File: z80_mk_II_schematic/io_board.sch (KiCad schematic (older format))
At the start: 3 parts

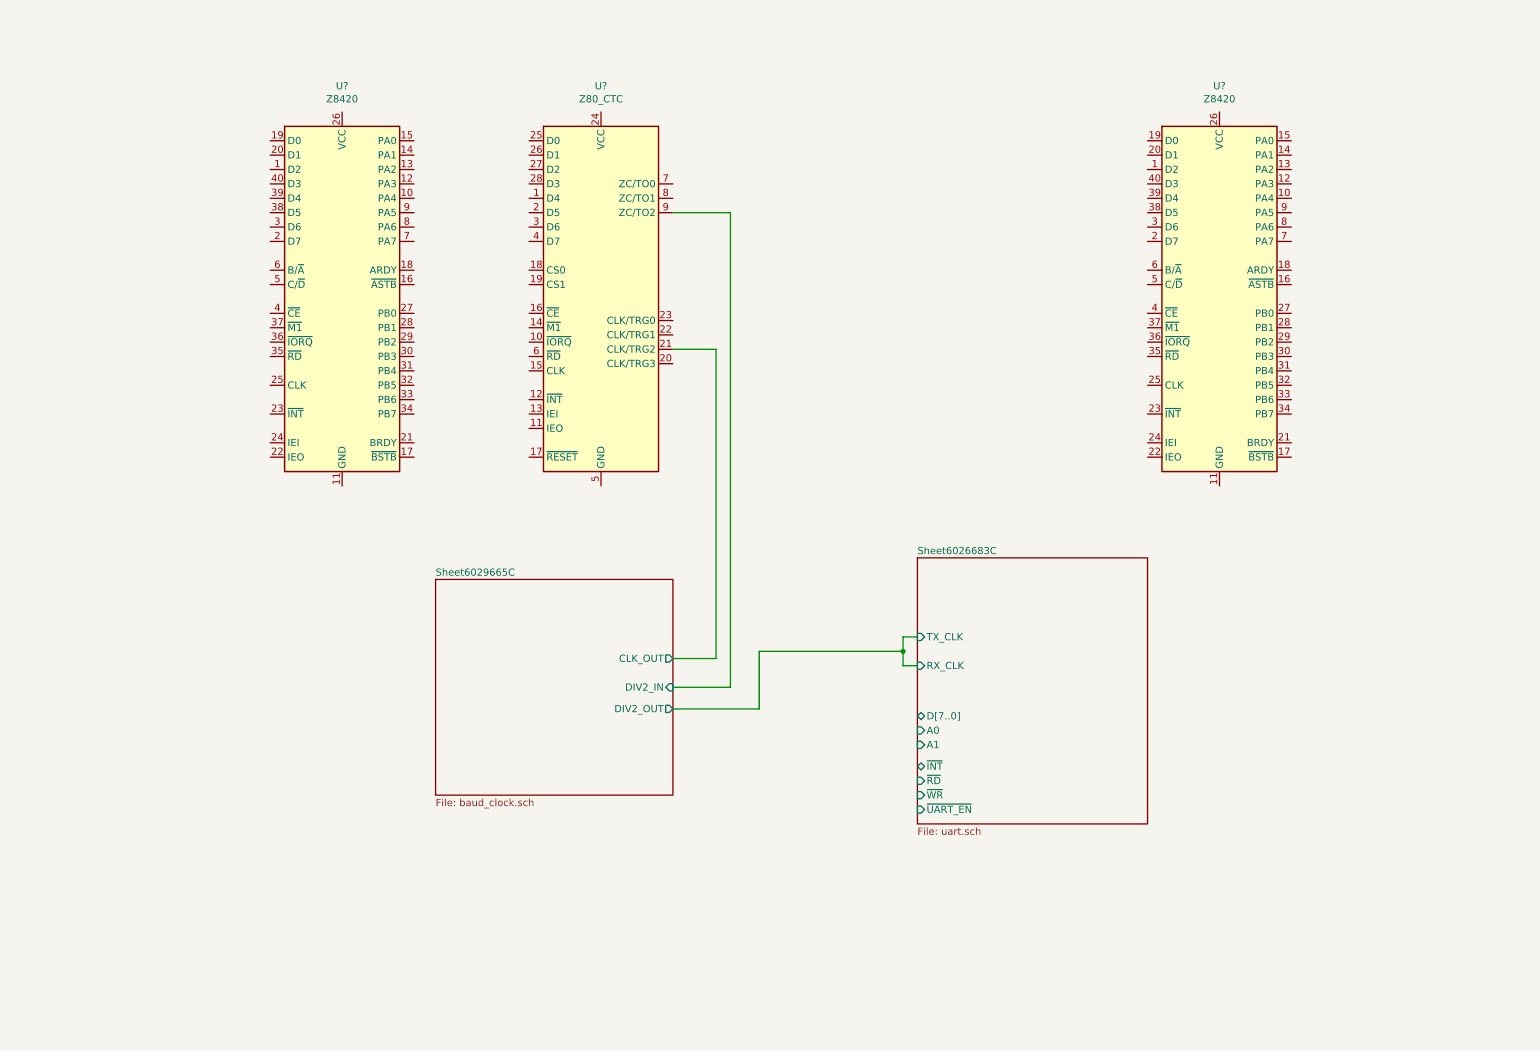
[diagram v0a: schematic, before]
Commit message: Lots more work on schematic
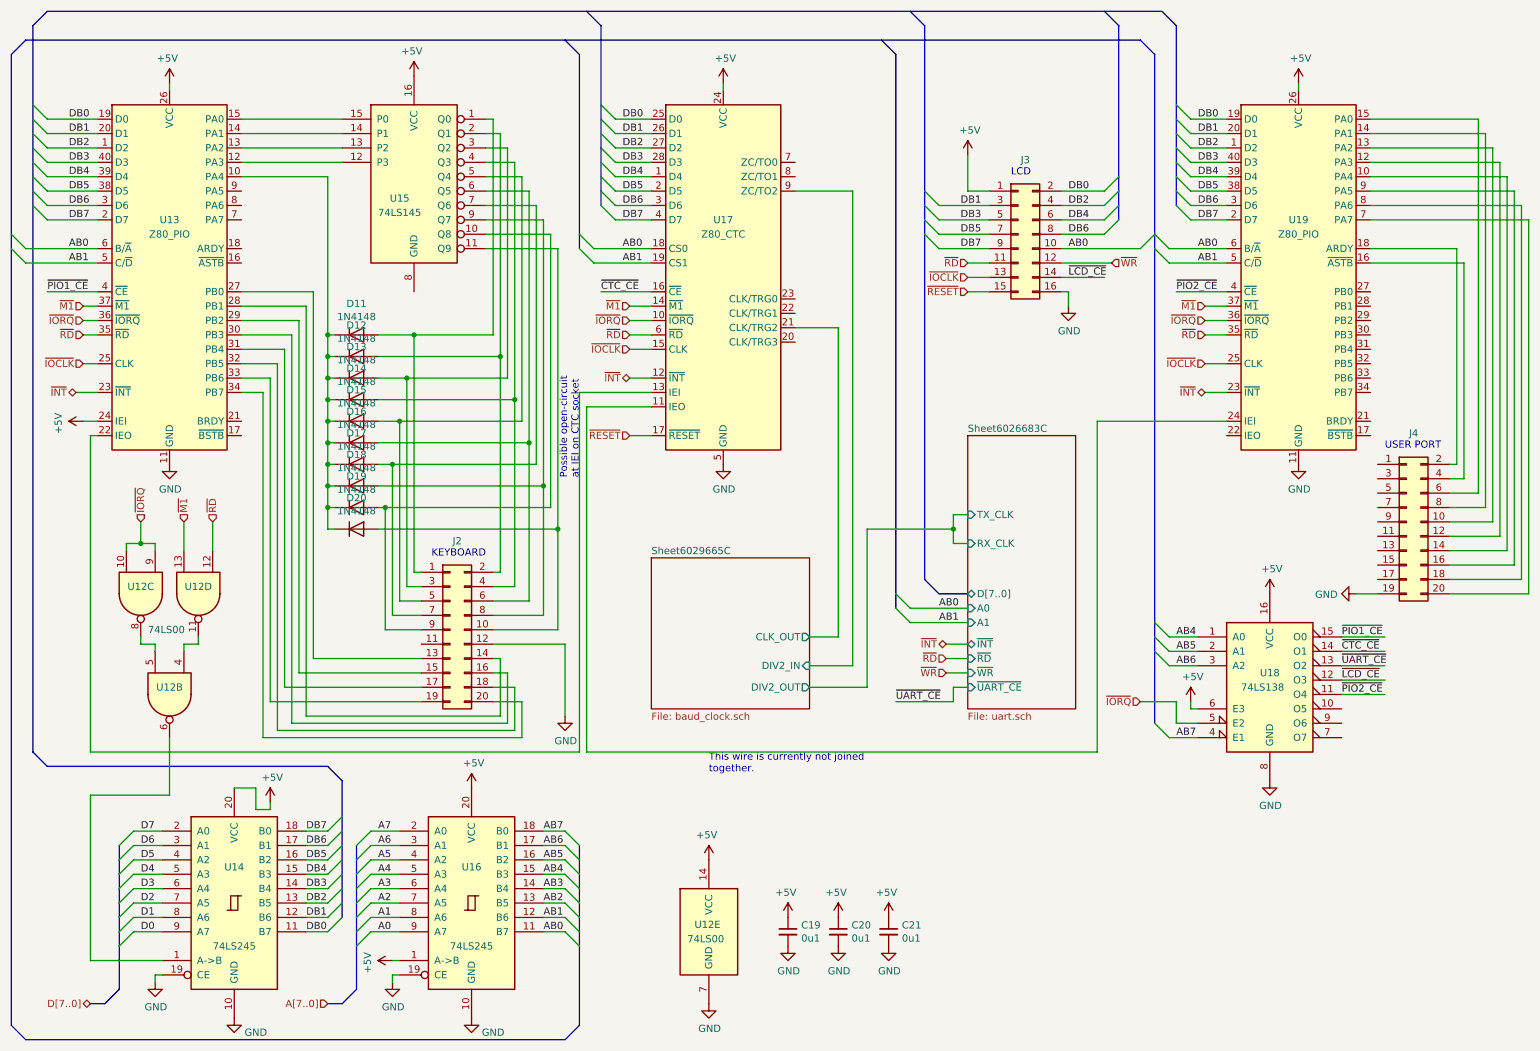
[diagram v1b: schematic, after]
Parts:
- added C19, C20, C21: 0u1, symbol Device:C_Small
- added D11, D12, D13, D14, D15, D16, D17, D18, D19, D20: 1N4148, Diode_THT:D_DO-35_SOD27_P7.62mm_Horizontal, symbol Diode:1N4148
- added J2, J4: Conn_02x10_Odd_Even, symbol Connector_Generic:Conn_02x10_Odd_Even
- added J3: Conn_02x08_Odd_Even, symbol Connector_Generic:Conn_02x08_Odd_Even
- added U12: 74LS00, symbol 74xx:74LS00
- added U14, U16: 74LS245, symbol 74xx:74LS245
- added U15: 74LS145, symbol 74xx:74LS145
- added U18: 74LS138, symbol 74xx:74LS138
- U13, U19: renamed from U?; value Z8420 -> Z80_PIO; footprint Package_DIP:DIP-40_W15.24mm -> (none)
- U17: renamed from U?; footprint Housings_DIP:DIP-28_W15.24mm -> (none)
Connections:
- net DB2: now reaches U13.1 (D2)
- net DB2: now also U17.27 (D2), U19.1 (D2), J3.4 (Pin_4), U14.13 (B5)
- net at U13.10 (PA4): now also D11.1 (K), D12.1 (K), D13.1 (K), D14.1 (K), D15.1 (K), D16.1 (K), D17.1 (K), D18.1 (K), D19.1 (K), D20.1 (K)
- net GND: now reaches U13.11 (GND)
- net GND: now also U17.5 (GND), U19.11 (GND), C19.2, C20.2, C21.2, J2.12 (Pin_12), J3.16 (Pin_16), J4.19 (Pin_19), U12.7 (GND), U14.10 (GND), U14.19 (CE), U16.10 (GND), U16.19 (CE), U18.8 (GND)
- net at U13.12 (PA3): now also U15.12 (P3)
- net at U13.13 (PA2): now also U15.13 (P2)
- net at U13.14 (PA1): now also U15.14 (P1)
- net at U13.15 (PA0): now also U15.15 (P0)
- net DB0: now reaches U13.19 (D0)
- net DB0: now also U17.25 (D0), U19.19 (D0), J3.2 (Pin_2), U14.11 (B7)
- net DB7: now reaches U13.2 (D7)
- net DB7: now also U17.4 (D7), U19.2 (D7), J3.9 (Pin_9), U14.18 (B0)
- net DB1: now reaches U13.20 (D1)
- net DB1: now also U17.26 (D1), U19.20 (D1), J3.3 (Pin_3), U14.12 (B6)
- net at U13.22 (IEO): now also U17.13 (IEI)
- net ~INT~: now reaches U13.23 (~INT~)
- net ~INT~: now also U17.12 (~INT~), U19.23 (~INT~)
- net +5V: now reaches U13.24 (IEI)
- net +5V: now also U13.26 (VCC), U17.24 (VCC), U19.26 (VCC), C19.1, C20.1, C21.1, J3.1 (Pin_1), U12.14 (VCC), U14.20 (VCC), U15.16 (VCC), U16.1 (A->B), U16.20 (VCC), U18.16 (VCC), U18.6 (E3)
- net ~IOCLK~: now reaches U13.25 (CLK)
- net ~IOCLK~: now also U17.15 (CLK), U19.25 (CLK), J3.13 (Pin_13)
- net at U13.27 (PB0): now also J2.13 (Pin_13)
- net at U13.28 (PB1): now also J2.14 (Pin_14)
- net at U13.29 (PB2): now also J2.15 (Pin_15)
- net DB6: now reaches U13.3 (D6)
- net DB6: now also U17.3 (D6), U19.3 (D6), J3.8 (Pin_8), U14.17 (B1)
- net at U13.30 (PB3): now also J2.16 (Pin_16)
- net at U13.31 (PB4): now also J2.17 (Pin_17)
- net at U13.32 (PB5): now also J2.18 (Pin_18)
- net at U13.33 (PB6): now also J2.19 (Pin_19)
- net at U13.34 (PB7): now also J2.20 (Pin_20)
- net ~RD~: now reaches U13.35 (~RD~)
- net ~RD~: now also U17.6 (~RD~), U19.35 (~RD~), J3.11 (Pin_11), U12.12
- net ~IORQ~: now reaches U13.36 (~IORQ~)
- net ~IORQ~: now also U17.10 (~IORQ~), U19.36 (~IORQ~), U12.10, U12.9, U18.5 (E2)
- net ~M1~: now reaches U13.37 (~M1~)
- net ~M1~: now also U17.14 (~M1~), U19.37 (~M1~), U12.13
- net DB5: now reaches U13.38 (D5)
- net DB5: now also U17.2 (D5), U19.38 (D5), J3.7 (Pin_7), U14.16 (B2)
- net DB4: now reaches U13.39 (D4)
- net DB4: now also U17.1 (D4), U19.39 (D4), J3.6 (Pin_6), U14.15 (B3)
- net ~PIO1_CE~: now reaches U13.4 (~CE~)
- net ~PIO1_CE~: now also U18.15 (O0)
- net DB3: now reaches U13.40 (D3)
- net DB3: now also U17.28 (D3), U19.40 (D3), J3.5 (Pin_5), U14.14 (B4)
- net AB1: now reaches U13.5 (C/~D~)
- net AB1: now also U17.19 (CS1), U19.5 (C/~D~), U16.12 (B6)
- net AB0: now reaches U13.6 (B/~A~)
- net AB0: now also U17.18 (CS0), U19.6 (B/~A~), J3.10 (Pin_10), U16.11 (B7)
- net at U19.10 (PA4): now also J4.14 (Pin_14)
- net at U19.12 (PA3): now also J4.12 (Pin_12)
- net at U19.13 (PA2): now also J4.10 (Pin_10)
- net at U19.14 (PA1): now also J4.8 (Pin_8)
- net at U19.15 (PA0): now also J4.6 (Pin_6)
- net at U19.16 (~ASTB~): now also J4.4 (Pin_4)
- net at U19.18 (ARDY): now also J4.2 (Pin_2)
- net at U19.24 (IEI): now also U17.11 (IEO)
- net ~PIO2_CE~: now reaches U19.4 (~CE~)
- net ~PIO2_CE~: now also U18.11 (O4)
- net at U19.7 (PA7): now also J4.20 (Pin_20)
- net at U19.8 (PA6): now also J4.18 (Pin_18)
- net at U19.9 (PA5): now also J4.16 (Pin_16)
- net ~CTC_CE~: now reaches U17.16 (~CE~)
- net ~CTC_CE~: now also U18.14 (O1)
- net ~RESET~: now reaches U17.17 (~RESET~)
- net ~RESET~: now also J3.15 (Pin_15)
- new net: D11.2 (A), J2.1 (Pin_1), U15.1 (Q0)
- new net: D20.2 (A), J2.10 (Pin_10), U15.11 (Q9)
- new net: D12.2 (A), J2.2 (Pin_2), U15.2 (Q1)
- new net: D13.2 (A), J2.3 (Pin_3), U15.3 (Q2)
- new net: D14.2 (A), J2.4 (Pin_4), U15.4 (Q3)
- new net: D15.2 (A), J2.5 (Pin_5), U15.5 (Q4)
- new net: D16.2 (A), J2.6 (Pin_6), U15.6 (Q5)
- new net: D17.2 (A), J2.7 (Pin_7), U15.7 (Q6)
- new net: D18.2 (A), J2.8 (Pin_8), U15.9 (Q7)
- new net: D19.2 (A), J2.9 (Pin_9), U15.10 (Q8)
- new net: U12.6, U14.1 (A->B)
- new net: U12.5, U12.8
- new net: U12.11, U12.4
- new net A0: U16.9 (A7)
- new net A1: U16.8 (A6)
- new net A2: U16.7 (A5)
- new net A3: U16.6 (A4)
- new net A4: U16.5 (A3)
- new net A5: U16.4 (A2)
- new net A6: U16.3 (A1)
- new net A7: U16.2 (A0)
- new net AB2: U16.13 (B5)
- new net AB3: U16.14 (B4)
- new net AB4: U16.15 (B3), U18.1 (A0)
- new net AB5: U16.16 (B2), U18.2 (A1)
- new net AB6: U16.17 (B1), U18.3 (A2)
- new net AB7: U16.18 (B0), U18.4 (E1)
- new net D0: U14.9 (A7)
- new net D1: U14.8 (A6)
- new net D2: U14.7 (A5)
- new net D3: U14.6 (A4)
- new net D4: U14.5 (A3)
- new net D5: U14.4 (A2)
- new net D6: U14.3 (A1)
- new net D7: U14.2 (A0)
- new net ~LCD_CE~: J3.14 (Pin_14), U18.12 (O3)
- new net ~UART_CE~: U18.13 (O2)
- new net ~WR~: J3.12 (Pin_12)
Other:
- note added: "KEYBOARD"
- note added: "LCD"
- note added: "Possible open-circuit\nat IEI on CTC socket"
- note added: "This wire is currently not joined\ntogether."
- note added: "USER PORT"
- moved on the sheet: U13, U17, U19
